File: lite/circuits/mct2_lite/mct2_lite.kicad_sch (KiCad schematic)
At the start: 4 parts

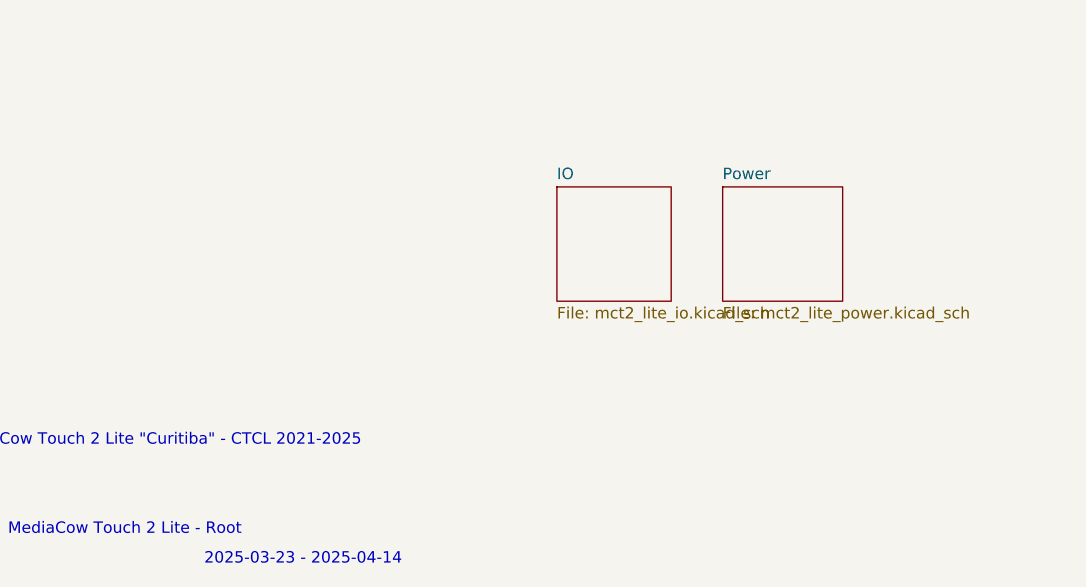
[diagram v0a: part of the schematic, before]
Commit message: 20250415-1
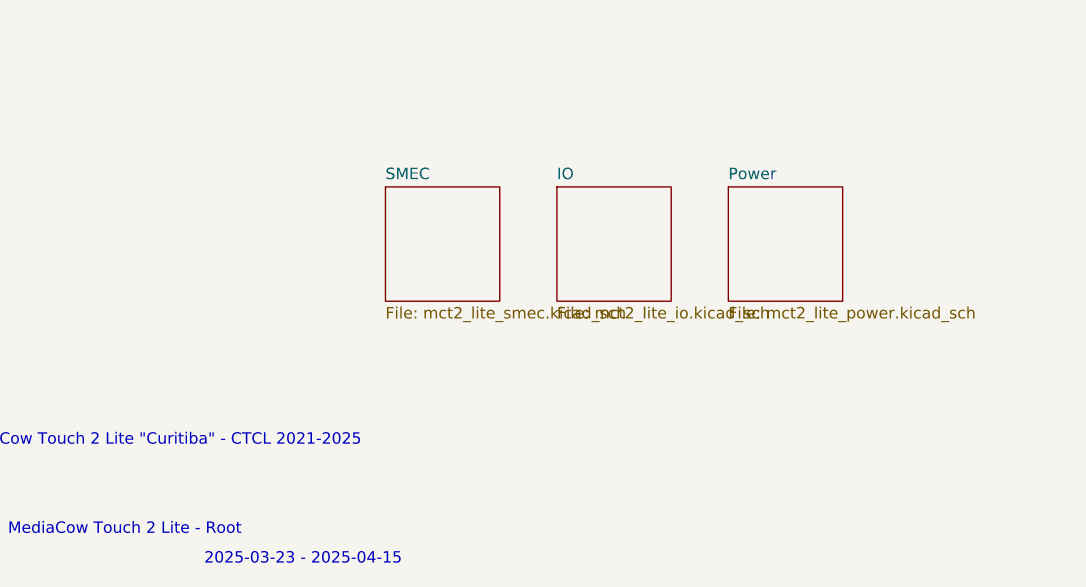
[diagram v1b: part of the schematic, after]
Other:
- added sheet SMEC (mct2_lite_smec.kicad_sch)
- note added: "2025-03-23 - 2025-04-15"
- note removed: "2025-03-23 - 2025-04-14"
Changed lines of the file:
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@@
 		)
 	)
-	(text "2025-03-23 - 2025-04-14"
+	(text "2025-03-23 - 2025-04-15"
 		(exclude_from_sim no)
 		(at 517.906 403.352 0)
@@
 	)
 	(sheet
+		(at 527.05 361.95)
+		(size 12.7 12.7)
+		(fields_autoplaced yes)
+		(stroke
+			(width 0.1524)
+			(type solid)
+		)
+		(fill
+			(color 0 0 0 0.0000)
+		)
+		(property "Sheetname" "SMEC"
+			(at 527.05 361.2384 0)
+			(effects
+				(font
+					(size 1.27 1.27)
+				)
+				(justify left bottom)
+			)
+		)
+		(property "Sheetfile" "mct2_lite_smec.kicad_sch"
+			(at 527.05 375.2346 0)
+			(effects
+				(font
+					(size 1.27 1.27)
+				)
+				(justify left top)
+			)
+		)
+		(instances
+			(project "mct2_lite"
+				(path "/caf0e9b0-a44c-4a4e-b706-dd9d72690bf9"
+					(page "4")
+				)
+			)
+		)
+	)
+	(sheet
 		(at 546.1 361.95)
 		(size 12.7 12.7)
@@
 	)
 	(sheet
-		(at 564.515 361.95)
-		(size 13.335 12.7)
+		(at 565.15 361.95)
+		(size 12.7 12.7)
 		(fields_autoplaced yes)
 		(stroke
@@
 		)
 		(property "Sheetname" "Power"
-			(at 564.515 361.2384 0)
+			(at 565.15 361.2384 0)
 			(effects
 				(font
@@
 		)
 		(property "Sheetfile" "mct2_lite_power.kicad_sch"
-			(at 564.515 375.2346 0)
+			(at 565.15 375.2346 0)
 			(effects
 				(font
